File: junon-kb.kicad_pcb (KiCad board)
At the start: 2 copper layers, 133 x 95 mm, 59 parts, among them IC1 BD41041FJ-CE2, J1 STLINK-V3MINIE, J2 SJ-43514-SMT-TR, J3 SJ-43514-SMT-TR, J4 632723300011, U1 STM32G473CCT3, U3 SPX3819M5-L-1-5/TR, Y1 ECS-3225MV-320-CN-TR

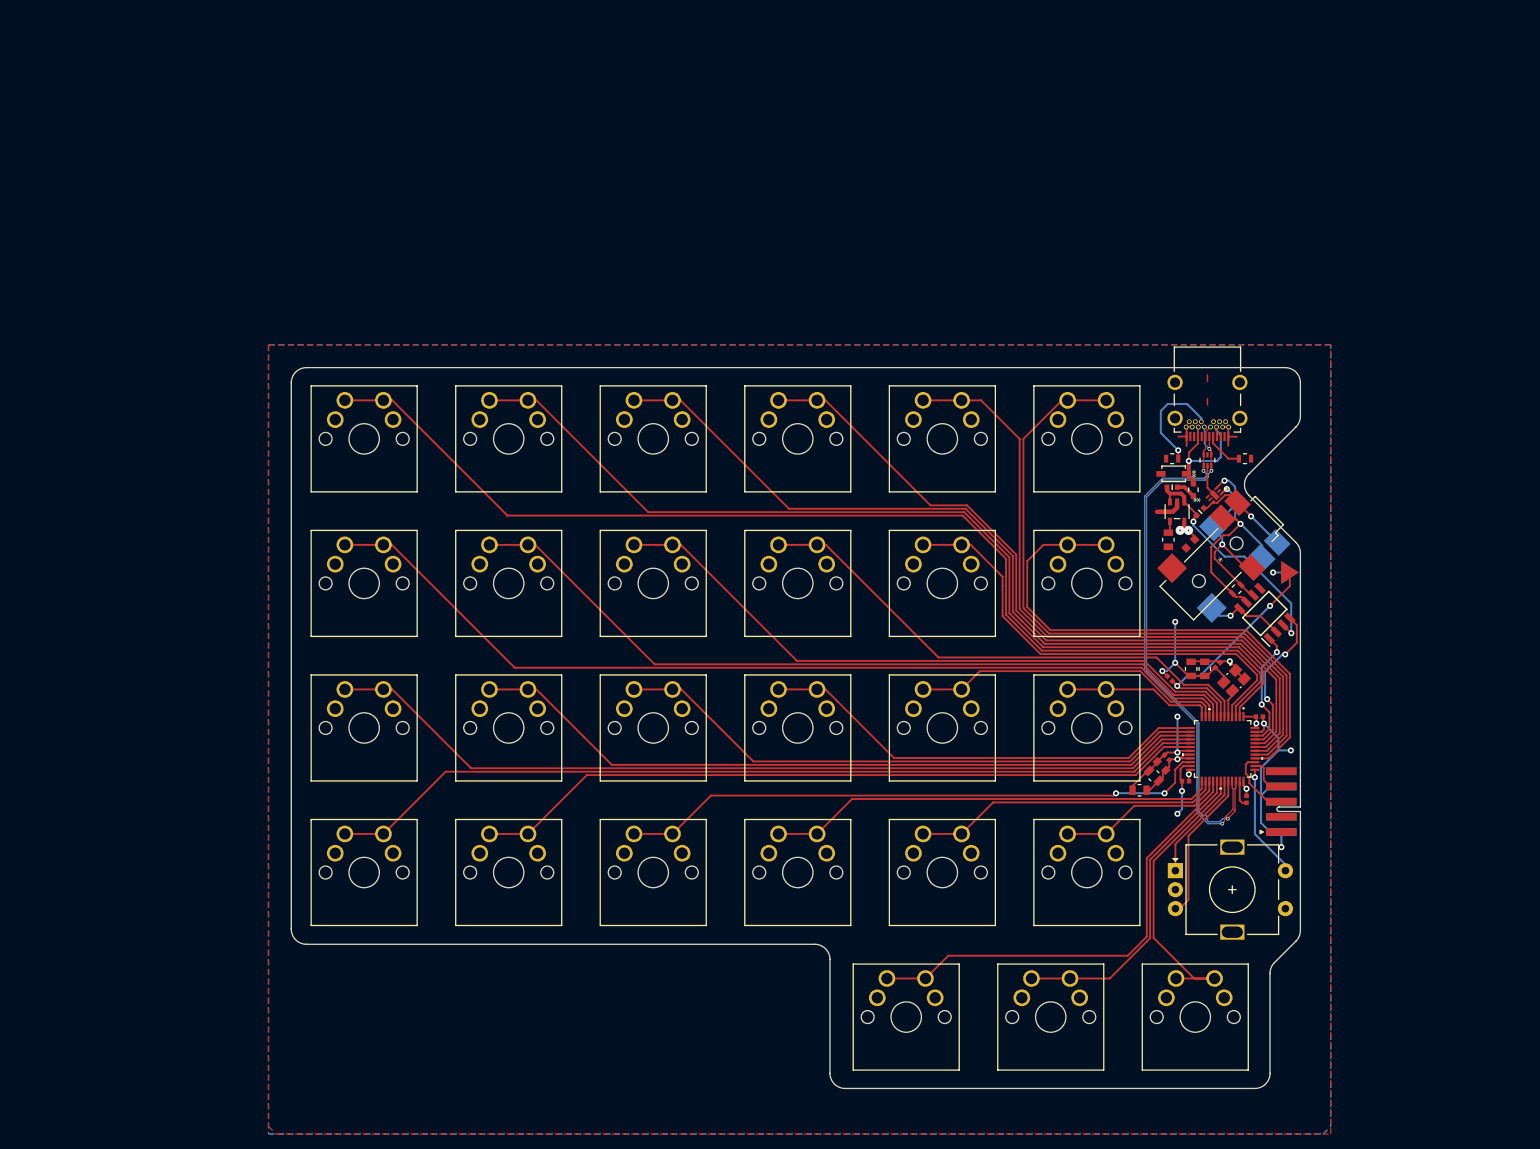
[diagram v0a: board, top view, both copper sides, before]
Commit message: more artifacts
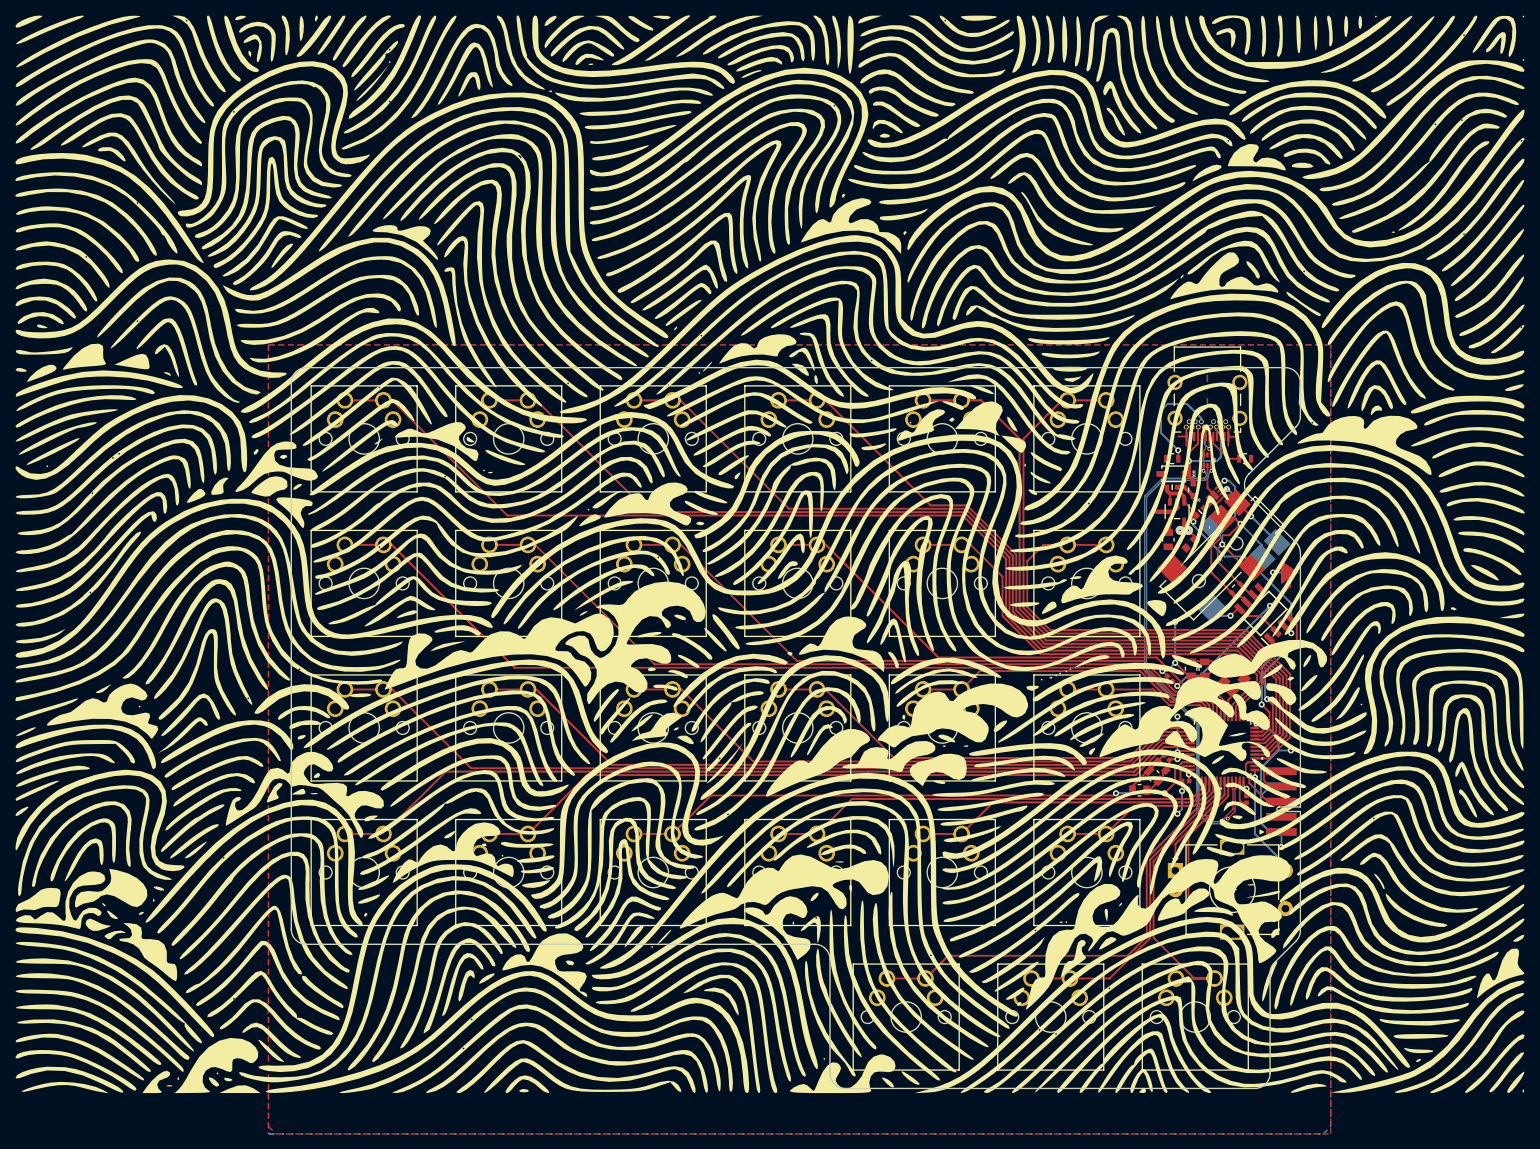
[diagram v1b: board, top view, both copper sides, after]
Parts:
- added G***: LOGO, LOGO, F.Cu at (131.1, 60.6)
- added G***: LOGO, LOGO, B.Cu at (164.6, 60.4)
